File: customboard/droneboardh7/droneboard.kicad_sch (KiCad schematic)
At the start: 59 parts, among them J1 Conn_01x04, J2 Conn_01x04, J3 Conn_01x05_Pin, J4 Conn_01x02_Pin, J5 USB_C_Receptacle_USB2.0_16P, J6 Conn_01x04, J7 Conn_01x01_Pin, J8 Conn_01x01_Pin, J9 Conn_01x01_Pin, SW1 SW_Push, SW2 SW_Push, U2 STM32H723VGTx, U3 LM7805MPX, U4 ICM-42688-P, U5 SPX3819M5-L-3-3, U6 SPX3819M5-L-3-3, Y2 CSTNE20M0V53Z000R0

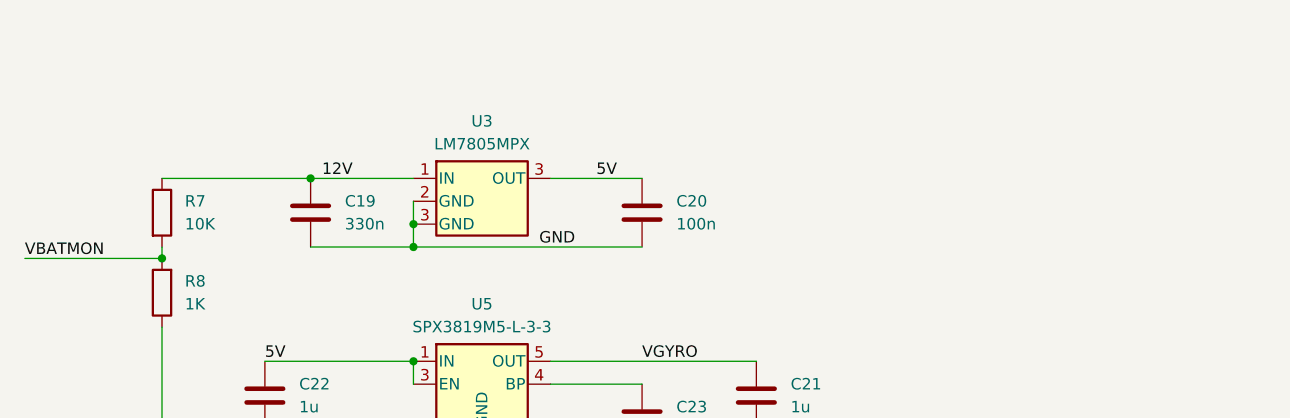
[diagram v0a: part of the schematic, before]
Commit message: smps initial
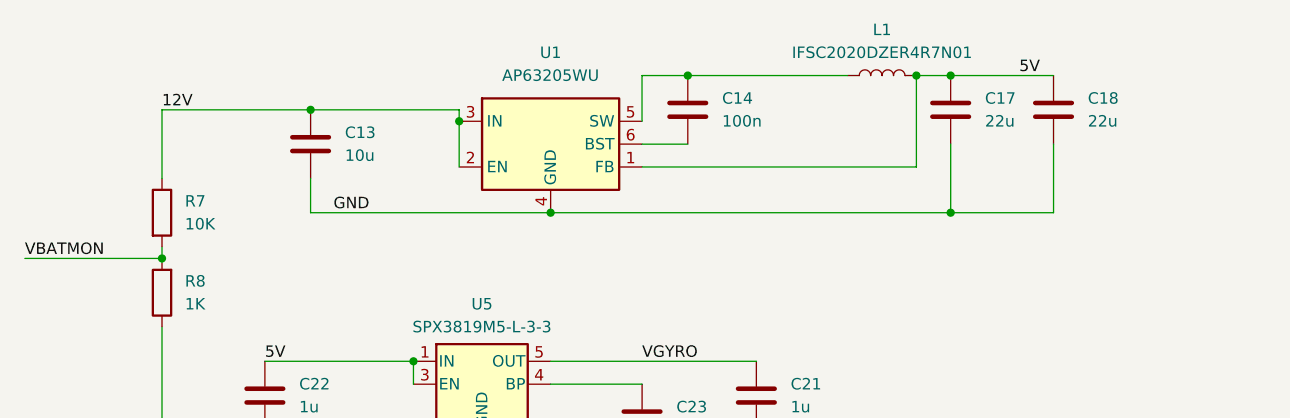
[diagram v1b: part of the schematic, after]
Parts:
- removed C19: 330n, Capacitor_SMD:C_0805_2012Metric, symbol Device:C
- removed C20: 100n, Capacitor_SMD:C_0603_1608Metric, symbol Device:C
- removed U3: LM7805MPX, Package_TO_SOT_SMD:SOT-223-3_TabPin2, symbol Regulator_Linear:L7805
- added C13: 10u, Capacitor_SMD:C_1206_3216Metric, symbol Device:C
- added C14: 100n, Capacitor_SMD:C_0603_1608Metric, symbol Device:C
- added C17, C18: 22u, Capacitor_SMD:C_0805_2012Metric, symbol Device:C
- added L1: IFSC2020DZER4R7N01, Inductor_SMD:L_Vishay_IHLP-2020, symbol Device:L
- added U1: AP63205WU, Package_TO_SOT_SMD:TSOT-23-6, symbol Regulator_Switching:AP63205WU
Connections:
- net 12V: now also C13.1, U1.2 (EN), U1.3 (IN)
- net 5V: now also C17.1, C18.1, L1.2, U1.1 (FB)
- net GND: now also C13.2, C17.2, C18.2, U1.4 (GND)
- new net: C14.1, U1.6 (BST)
- new net: C14.2, L1.1, U1.5 (SW)
